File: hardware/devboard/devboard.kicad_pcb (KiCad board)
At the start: 2 copper layers, 52 x 71.5 mm, 49 parts, among them J1 10103594-0001LF, J2 TSW-126-07-L-D, J3 TSW-126-07-L-D, J4 SM03B-SRSS-TB(LF)(SN), SW1 434133025816, SW2 434133025816, U1 RP2350B, U2 NCP1117ST33T3G, U3 W25Q128JVSIQ, U4 W25Q128JVSIQ, X1 12MHz

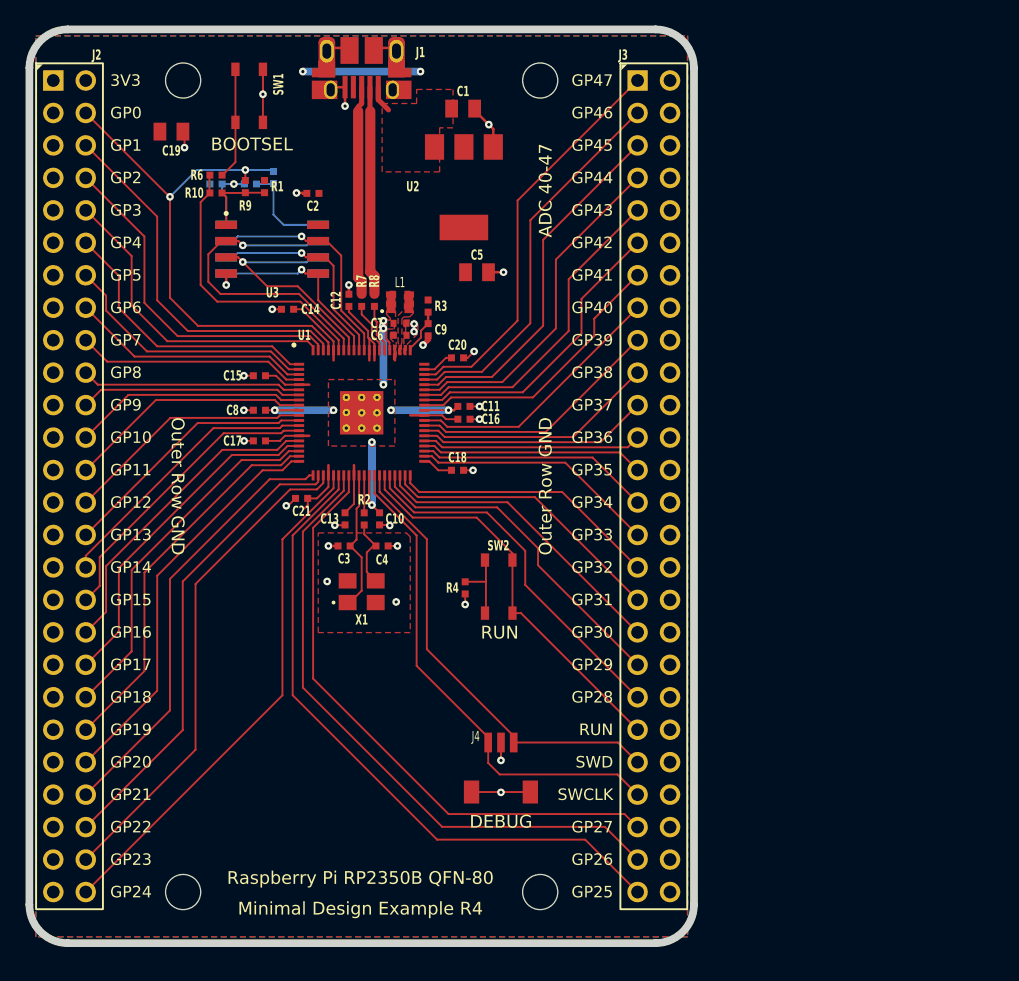
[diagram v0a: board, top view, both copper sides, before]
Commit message: feat(pcb): add first PCB for the devboard
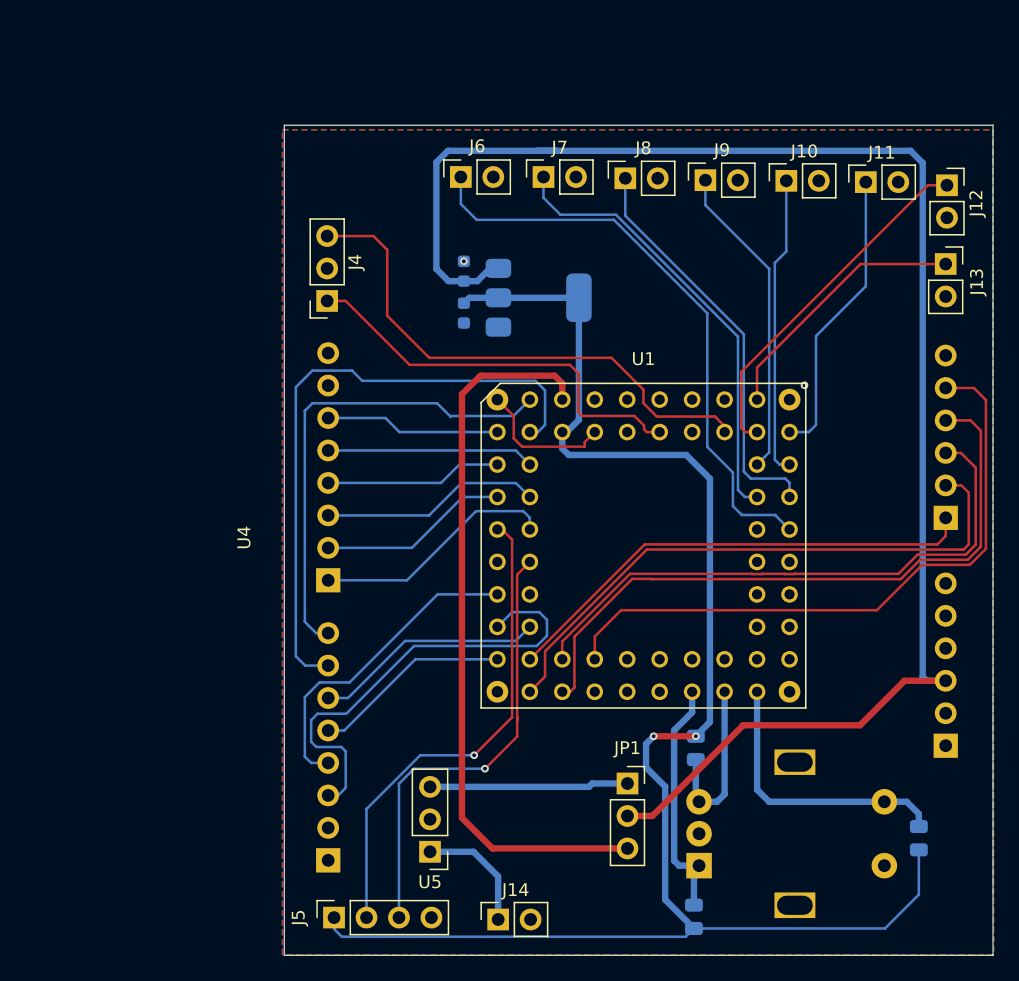
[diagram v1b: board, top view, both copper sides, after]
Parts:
- removed C10, C11, C12, C13, C14, C15, C16, C17, C18, C2, C20, C21, C22, C8: 100n, RPI_COMPILED:generic_capc1005x50
- removed C19: 10u, RPI_COMPILED:generic_capc2012x125
- removed C3, C4: 15p, RPI_COMPILED:generic_capc1005x50
- removed C6, C7: 4.7u, RPI_COMPILED:generic_capc1005x50_wide
- removed C9: 4.7u, RPI_COMPILED:generic_capc1005x50
- removed J1: 10103594-0001LF, RPI_COMPILED:amphenol_10103594-0001lf
- removed J2, J3: TSW-126-07-L-D, RPI_COMPILED:samtec_tsw-126-07-l-d
- removed L1: 3.3u, RPI_COMPILED:abracon_aota-b201610s3r3-101-t
- removed MH1, MH2, MH3, MH4: NPTH FD2.75mm SM3.15mm KO6mm, RPI_COMPILED:none_mh_npth_fd2p75mm_sm3p15mm_ko6mm
- removed R10, R11, R9: 0, RPI_COMPILED:generic_resc1005x35
- removed R13: 10k, RPI_COMPILED:generic_resc1005x35
- removed R4, R6: 1k, RPI_COMPILED:generic_resc1005x35
- removed R7, R8: 27, RPI_COMPILED:generic_resc1005x35
- removed SW2: 434133025816, RPI_COMPILED:wurthelek_434133025816
- removed U3: W25Q128JVSIQ, RPI_COMPILED:generic_soic127p790x195-8
- removed X1: 12MHz, RPI_COMPILED:generic_xtalcc320x250x80-4
- added J10: ADC4, Connector_PinSocket_2.54mm:PinSocket_1x02_P2.54mm_Vertical, F.Cu at (133.2, 81.8)
- added J11: ADC5, Connector_PinSocket_2.54mm:PinSocket_1x02_P2.54mm_Vertical, F.Cu at (139.4, 82.0)
- added J12: ADC6, Connector_PinSocket_2.54mm:PinSocket_1x02_P2.54mm_Vertical, F.Cu at (145.8, 82.2)
- added J13: ADC7, Connector_PinSocket_2.54mm:PinSocket_1x02_P2.54mm_Vertical, F.Cu at (145.7, 88.4)
- added J14: Conn_01x02, Connector_PinSocket_2.54mm:PinSocket_1x02_P2.54mm_Vertical, F.Cu at (110.7, 139.7)
- added J5: I2C, Connector_PinSocket_2.54mm:PinSocket_1x04_P2.54mm_Vertical, F.Cu at (97.8, 139.5)
- added J6: ADC0, Connector_PinSocket_2.54mm:PinSocket_1x02_P2.54mm_Vertical, F.Cu at (107.8, 81.5)
- added J7: ADC1, Connector_PinSocket_2.54mm:PinSocket_1x02_P2.54mm_Vertical, F.Cu at (114.2, 81.5)
- added J8: ADC2, Connector_PinSocket_2.54mm:PinSocket_1x02_P2.54mm_Vertical, F.Cu at (120.6, 81.7)
- added J9: ADC3, Connector_PinSocket_2.54mm:PinSocket_1x02_P2.54mm_Vertical, F.Cu at (126.9, 81.8)
- added JP1: Jumper_3_Bridged12, Connector_PinSocket_2.54mm:PinSocket_1x03_P2.54mm_Vertical, F.Cu at (120.8, 129.0)
- added U5: ~, Connector_PinHeader_2.54mm:PinHeader_1x03_P2.54mm_Vertical, F.Cu at (105.3, 134.3)
- C1, C5: footprint RPI_COMPILED:generic_capc2012x125 -> Capacitor_SMD:C_0603_1608Metric; moved to B.Cu
- J4: value SM03B-SRSS-TB(LF)(SN) -> Conn_01x03; footprint RPI_COMPILED:jst_sm03b-srss-tb-lf--sn- -> Connector_PinSocket_2.54mm:PinSocket_1x03_P2.54mm_Vertical
- R1: footprint RPI_COMPILED:generic_resc1005x35 -> Resistor_SMD:R_0805_2012Metric; moved to B.Cu
- R2: value 1k -> 10k; footprint RPI_COMPILED:generic_resc1005x35 -> Resistor_SMD:R_0805_2012Metric; moved to B.Cu
- R3: value 33 -> 10k; footprint RPI_COMPILED:generic_resc1005x35 -> Resistor_SMD:R_0805_2012Metric; moved to B.Cu
- SW1: value 434133025816 -> RotaryEncoder_Switch_MP; footprint RPI_COMPILED:wurthelek_434133025816 -> Rotary_Encoder:RotaryEncoder_Alps_EC11E-Switch_Vertical_H20mm; moved to B.Cu
- U1: value RP2350B -> Core2350B0; footprint RPI_COMPILED:rpi_rp2350b_vias -> Project Library:Core2350B0
- U2: value NCP1117ST33T3G -> AMS1117CD-3.3; footprint RPI_COMPILED:onsemi_ncp1117st33t3g -> Package_TO_SOT_SMD:SOT-223-3_TabPin2; moved to B.Cu
- U4: value W25Q128JVSIQ -> ILI9486_35_Shield; footprint RPI_COMPILED:generic_soic127p790x195-8 -> Project Library:ILI9486_35_Shield; moved to F.Cu
- moved SW1 69.8 mm to (126.4, 135.4), turned to 0 degrees
- moved R1 66.3 mm to (126.0, 139.4), turned to 90 degrees
- moved U4 64.3 mm to (93.8, 151.5), turned to 90 degrees
- moved R3 56.6 mm to (143.6, 133.3), turned to 90 degrees
- moved J4 41.4 mm to (97.3, 91.2), turned to 180 degrees
- moved R2 31.5 mm to (126.2, 126.2)
- moved U1 24.4 mm to (122.0, 110.4)
- moved C1 12.7 mm to (108.0, 88.9), turned to 90 degrees
- moved U2 10.4 mm to (113.8, 91.0), turned to 0 degrees
- moved C5 3.36 mm to (108.0, 92.2), turned to -90 degrees
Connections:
- C1 pad 1: VBUS -> VSYS
- R1 pad 2: /FLASH_SS -> /GPIO27
- R2 pad 1: /XOUT -> +3V3
- R2 pad 2: Net-(C4-Pad1) -> /GPIO29
- R3 pad 2: /VREG_AVDD -> /GPIO30
- U1 pad 1: /GPIO4 -> /GPIO1
- U1 pad 10: +1V1 -> /GPIO10
- U1 pad 11: /GPIO12 -> /GPIO11
- U1 pad 12: /GPIO13 -> /GPIO12
- U1 pad 13: /GPIO14 -> /GPIO13
- U1 pad 14: /GPIO15 -> /GPIO14
- U1 pad 15: +3V3 -> /GPIO15
- U1 pad 2: /GPIO5 -> /GPIO2
- U1 pad 24: +3V3 -> /GPIO24
- U1 pad 25: /GPIO24 -> /GPIO25
- U1 pad 26: /GPIO25 -> /GPIO26
- U1 pad 27: /GPIO26 -> /GPIO27
- U1 pad 28: /GPIO27 -> /GPIO28
- U1 pad 29: +3V3 -> /GPIO29
- U1 pad 3: /GPIO6 -> /GPIO3
- U1 pad 30: /XIN -> /GPIO30
- U1 pad 31: /XOUT -> /GPIO31
- U1 pad 32: +1V1 -> /GPIO32
- U1 pad 33: /SWCLK -> /GPIO33
- U1 pad 34: /SWD -> /GPIO34
- U1 pad 35: /RUN -> /GPIO35
- U1 pad 36: /GPIO28 -> /GPIO36
- U1 pad 37: /GPIO29 -> /GPIO37
- U1 pad 38: /GPIO30 -> /GPIO38
- U1 pad 39: /GPIO31 -> /GPIO39
- U1 pad 4: /GPIO7 -> /GPIO4
- U1 pad 40: /GPIO32 -> /GPIO40_ADC0
- U1 pad 41: +3V3 -> /GPIO41_ADC1
- U1 pad 42: /GPIO33 -> /GPIO42_ADC2
- U1 pad 43: /GPIO34 -> /GPIO43_ADC3
- U1 pad 44: /GPIO35 -> /GPIO44_ADC4
- U1 pad 45: /GPIO36 -> /GPIO45_ADC5
- U1 pad 46: /GPIO37 -> /GPIO46_ADC6
- U1 pad 47: /GPIO38 -> /GPIO47_ADC7
- U1 pad 5: +3V3 -> /GPIO5
- U1 pad 6: /GPIO8 -> /GPIO6
- U1 pad 7: /GPIO9 -> /GPIO7
- U1 pad 8: /GPIO10 -> /GPIO8
- U1 pad 9: /GPIO11 -> /GPIO9
- U2 pad 3: VBUS -> VSYS
- U4 pad 1: /FLASH2_SS -> unconnected-(U4-NC-Pad1)
- U4 pad 2: /QSPI_SD1 -> unconnected-(U4-NC-Pad2)
- U4 pad 3: /QSPI_SD2 -> /GPIO14
- U4 pad 4: GND -> /GPIO12
- U4 pad 5: /QSPI_SD0 -> /GPIO15
- U4 pad 6: /QSPI_SCLK -> /GPIO13
- U4 pad 7: /QSPI_SD3 -> /GPIO1
- U4 pad 8: +3V3 -> /GPIO0
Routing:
- net VSYS: track 0.00 -> 125.7 mm
- net +3V3: track 52.9 -> 126.8 mm, vias 3 -> 2
- net VBUS: track 2.11 -> 57.1 mm
- net /GPIO25: track 52.1 -> 0.00 mm
- net /GPIO26: track 49.7 -> 0.00 mm
- net /GPIO24: track 40.6 -> 0.00 mm
- net /GPIO23: track 39.0 -> 0.00 mm
- net /GPIO22: track 36.7 -> 0.00 mm
- net /GPIO21: track 34.2 -> 0.00 mm
- net /RUN: track 31.4 -> 0.00 mm
- net +1V1: track 30.2 -> 0.00 mm, vias 9 -> 0
- net /GPIO28: track 28.7 -> 0.00 mm
- net /GPIO27: track 47.3 -> 19.2 mm
- net GND: track 38.8 -> 10.8 mm, vias 29 -> 2
- net /GPIO40_ADC0: track 20.8 -> 46.1 mm
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- removed copper zone on F.Cu, net +1V1
- removed copper zone on F.Cu, net +3V3
- removed copper zone on F.Cu, net /VREG_LX
- removed copper zone on F.Cu, net VBUS
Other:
- board size 52 x 71.5 mm -> 55.5 x 64.9 mm
- board text removed: "3V3"
- board text removed: "ADC 40-47"
- board text removed: "BOOTSEL"
- board text removed: "DEBUG"
- board text removed: "GP0"
- board text removed: "GP1"
- board text removed: "GP10"
- board text removed: "GP11"
- board text removed: "GP12"
- board text removed: "GP13"
- board text removed: "GP14"
- board text removed: "GP15"
- board text removed: "GP16"
- board text removed: "GP17"
- board text removed: "GP18"
- board text removed: "GP19"
- board text removed: "GP2"
- board text removed: "GP20"
- board text removed: "GP21"
- board text removed: "GP22"
- board text removed: "GP23"
- board text removed: "GP24"
- board text removed: "GP25"
- board text removed: "GP26"
- board text removed: "GP27"
- board text removed: "GP28"
- board text removed: "GP29"
- board text removed: "GP3"
- board text removed: "GP30"
- board text removed: "GP31"
- board text removed: "GP32"
- board text removed: "GP33"
- board text removed: "GP34"
- board text removed: "GP35"
- board text removed: "GP36"
- board text removed: "GP37"
- board text removed: "GP38"
- board text removed: "GP39"
- board text removed: "GP4"
- board text removed: "GP40"
- board text removed: "GP41"
- board text removed: "GP42"
- board text removed: "GP43"
- board text removed: "GP44"
- board text removed: "GP45"
- board text removed: "GP46"
- board text removed: "GP47"
- board text removed: "GP5"
- board text removed: "GP6"
- board text removed: "GP7"
- board text removed: "GP8"
- board text removed: "GP9"
- board text removed: "Minimal Design Example R4"
- board text removed: "Outer Row GND"
- board text removed: "RUN"
- board text removed: "Raspberry Pi RP2350B QFN-80"
- board text removed: "SWCLK"
- board text removed: "SWD"
